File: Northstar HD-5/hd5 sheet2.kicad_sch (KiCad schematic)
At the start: 69 parts, among them U1A1 26LS32, U1C1 74S10, U1D1 74S00, U1F1 74S04, U1H1 74LS123, U2A1 100ns_Delay, U2B1 74LS161, U2C1 74LS74, U2H1 74LS283, U2J1 74LS393, U3A1 74S74, U3B1 74S02, U3C1 74LS161, U3D1 74LS04, U3E1 74LS161, U3F1 74LS393, U3H1 74LS273, U3J1 74LS193, U4A1 74S74, U4B1 74S02, U4C1 74S74, U4D1 74S04, U4F1 74LS193, U4H1 74LS193, U4J1 74LS04, U5D1 74S124, U5F1 74S74, U5H1 74LS32, U5J1 74LS00, U5K1 74LS279

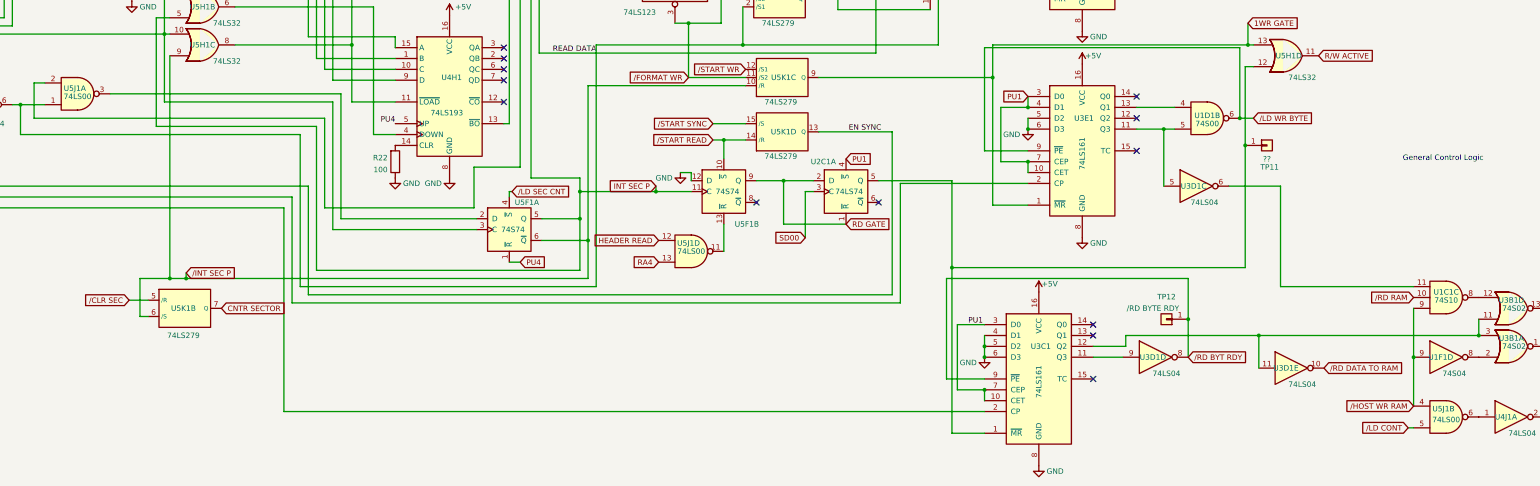
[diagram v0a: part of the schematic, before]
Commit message: small updates to boards
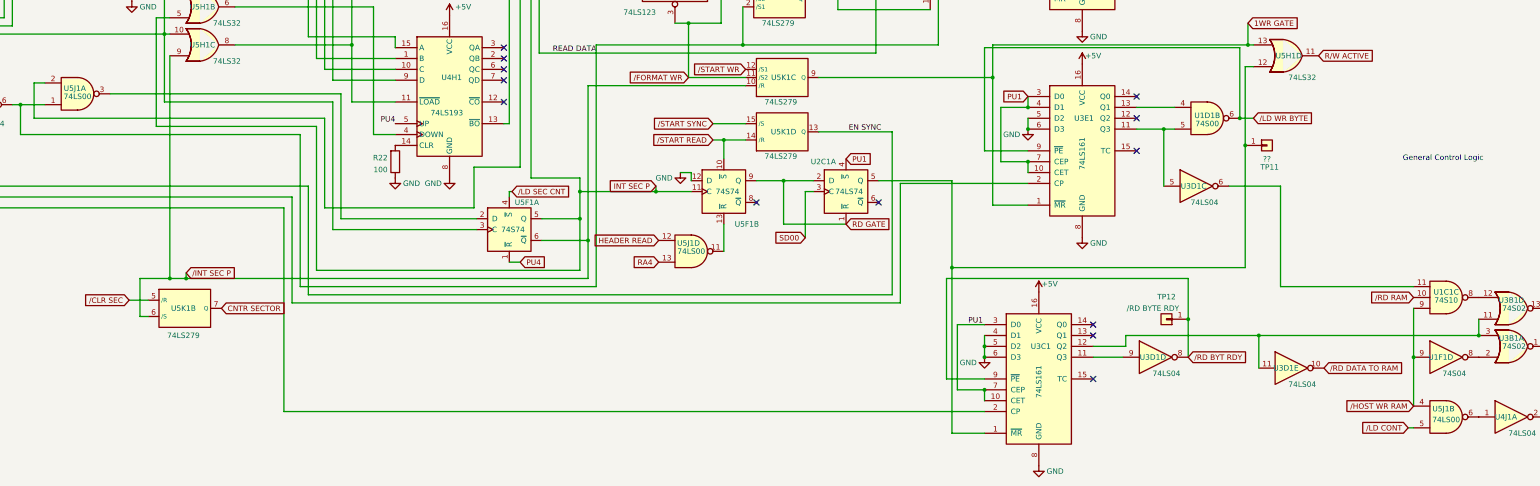
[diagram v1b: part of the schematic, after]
